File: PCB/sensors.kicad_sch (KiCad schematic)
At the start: 6 parts, among them J12 R-INMP441, J13 L-INMP441, J15 F_HS-SR04+, J16 B_HS-SR04+, J17 MPU-6050, U12 Module-3

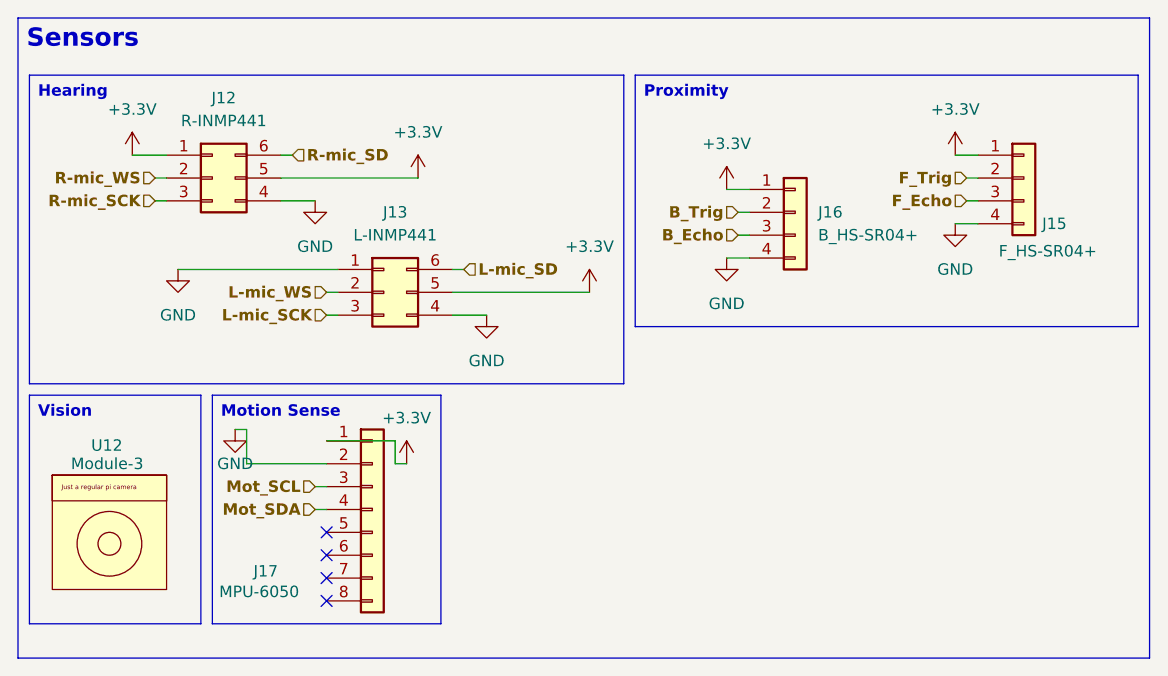
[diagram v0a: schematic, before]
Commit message: [PCB] Assigned all the footprints
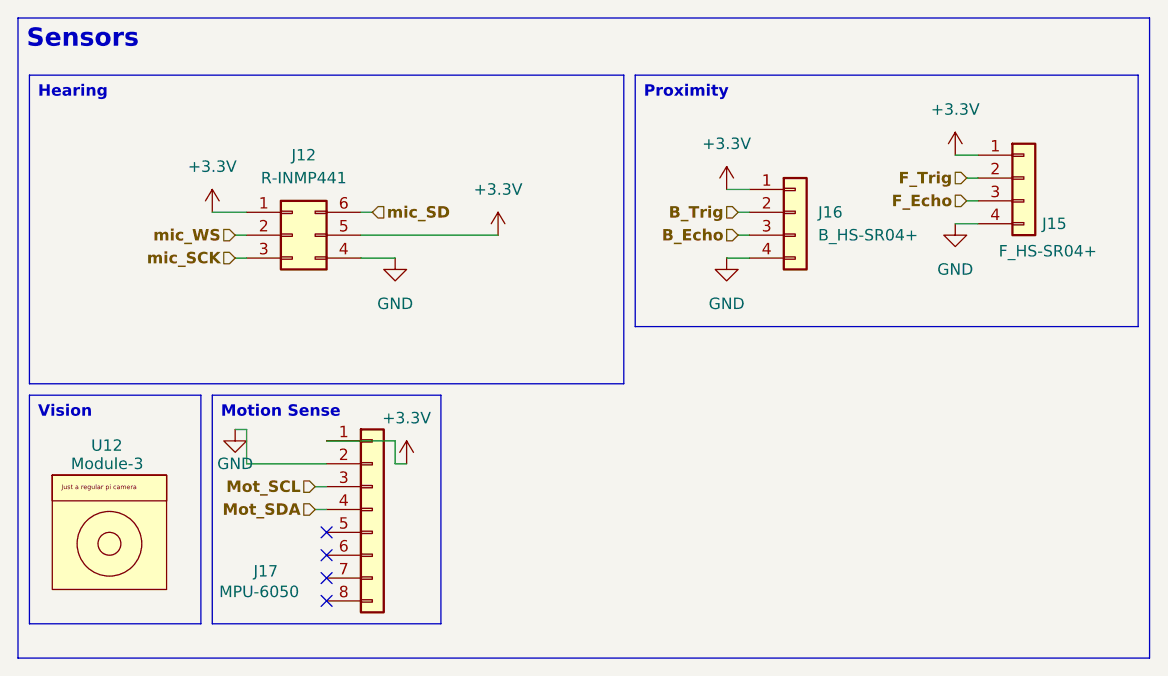
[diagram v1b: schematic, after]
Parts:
- removed J13: L-INMP441, symbol Connector_Generic:Conn_02x03_Counter_Clockwise
- J12: footprint (none) -> Connector_JST:JST_ZH_B6B-ZR-SM4-TF_1x06-1MP_P1.50mm_Vertical
- J15, J16: footprint (none) -> Connector_JST:JST_ZH_B4B-ZR-SM4-TF_1x04-1MP_P1.50mm_Vertical
- J17: footprint (none) -> Connector_JST:JST_ZH_B8B-ZR-SM4-TF_1x08-1MP_P1.50mm_Vertical
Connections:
- net R-mic_SCK renamed mic_SCK
- net R-mic_SD renamed mic_SD
- net R-mic_WS renamed mic_WS
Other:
- moved on the sheet: J12
